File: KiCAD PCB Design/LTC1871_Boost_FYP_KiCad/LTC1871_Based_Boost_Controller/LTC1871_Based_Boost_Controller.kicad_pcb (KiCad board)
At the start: 2 copper layers, 59.5 x 40 mm, 35 parts, among them J2 J2_OUT, J3 Proto_GND, J4 Proto_1, J5 Proto_2, Q1 IRF7811, Q2 DMP3099L, U1 LTC1871EMS-7-PBF

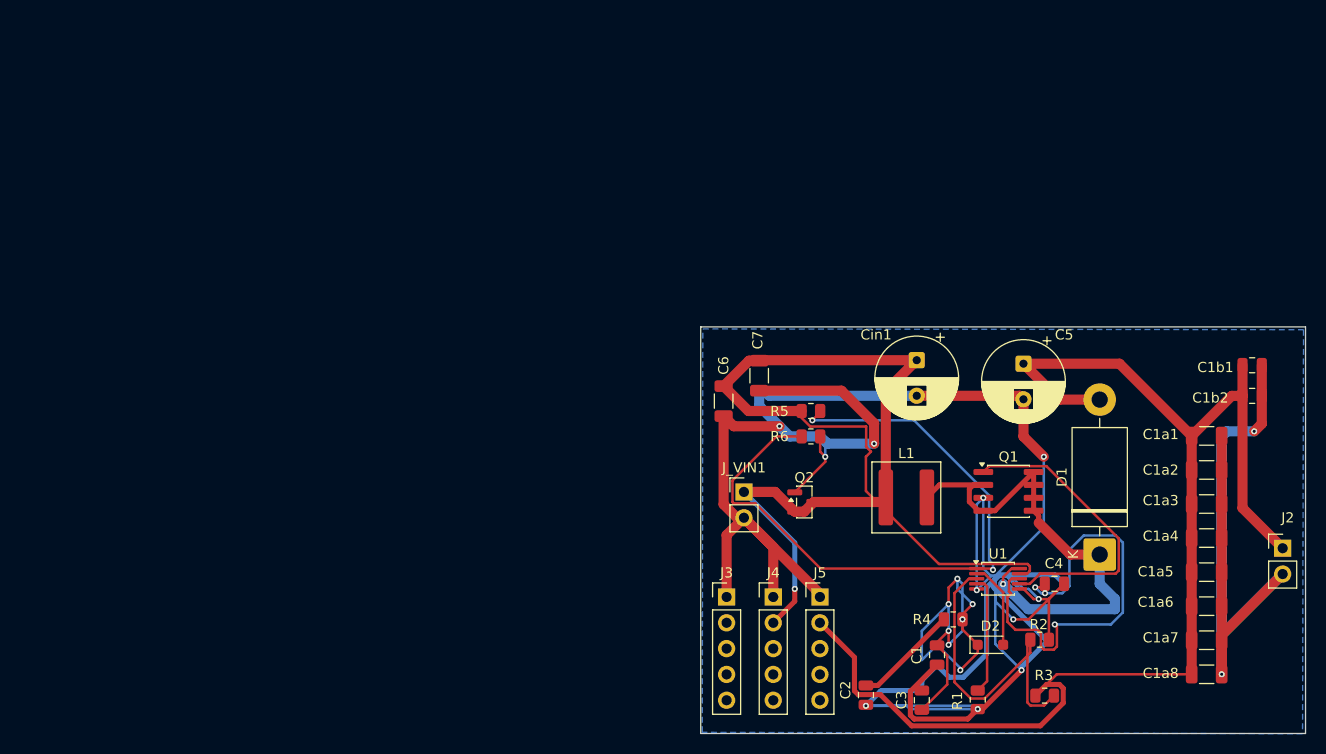
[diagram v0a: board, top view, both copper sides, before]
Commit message: Auto-sync from Fortune at 2026-04-10 17:12:48
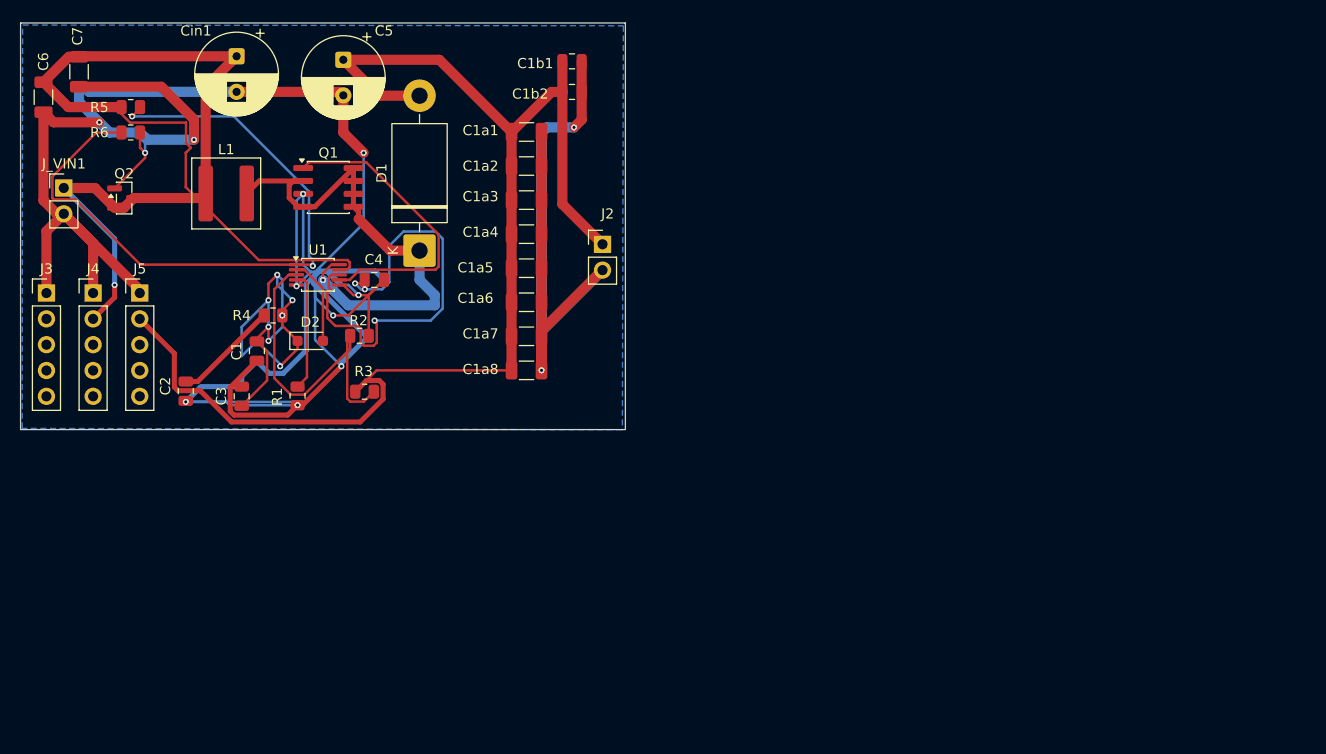
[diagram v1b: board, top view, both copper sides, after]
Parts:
- moved C4 73.3 mm to (142.1, 99.6)
- moved R5 73.3 mm to (118.2, 82.6)
- moved R6 73.3 mm to (118.2, 85.1)
- moved C1 73.3 mm to (130.6, 106.6)
- moved C1a1 73.3 mm to (157.1, 85.0)
- moved C1a2 73.3 mm to (157.1, 88.4)
- moved C1a3 73.3 mm to (157.1, 91.8)
- moved C1a4 73.3 mm to (157.1, 95.1)
- moved C1a5 73.3 mm to (157.1, 98.5)
- moved C1a6 73.3 mm to (157.1, 101.8)
- moved C1a7 73.3 mm to (157.1, 105.2)
- moved C1a8 73.3 mm to (157.1, 108.5)
- moved C1b1 73.3 mm to (161.6, 78.1)
- moved C1b2 73.3 mm to (161.6, 81.1)
- moved C2 73.3 mm to (123.6, 110.5)
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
